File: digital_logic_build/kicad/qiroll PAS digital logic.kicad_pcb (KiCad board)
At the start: 2 copper layers, 49.5 x 32.4 mm, 47 parts, among them J2 led_sw1, J3 accessory, J4 mode_thr_batt, J5 3_pin, U1 4093B, U2 4027B, U3 4093B, U5 4093B, U6 14538B, U7 MCP1799_3V3

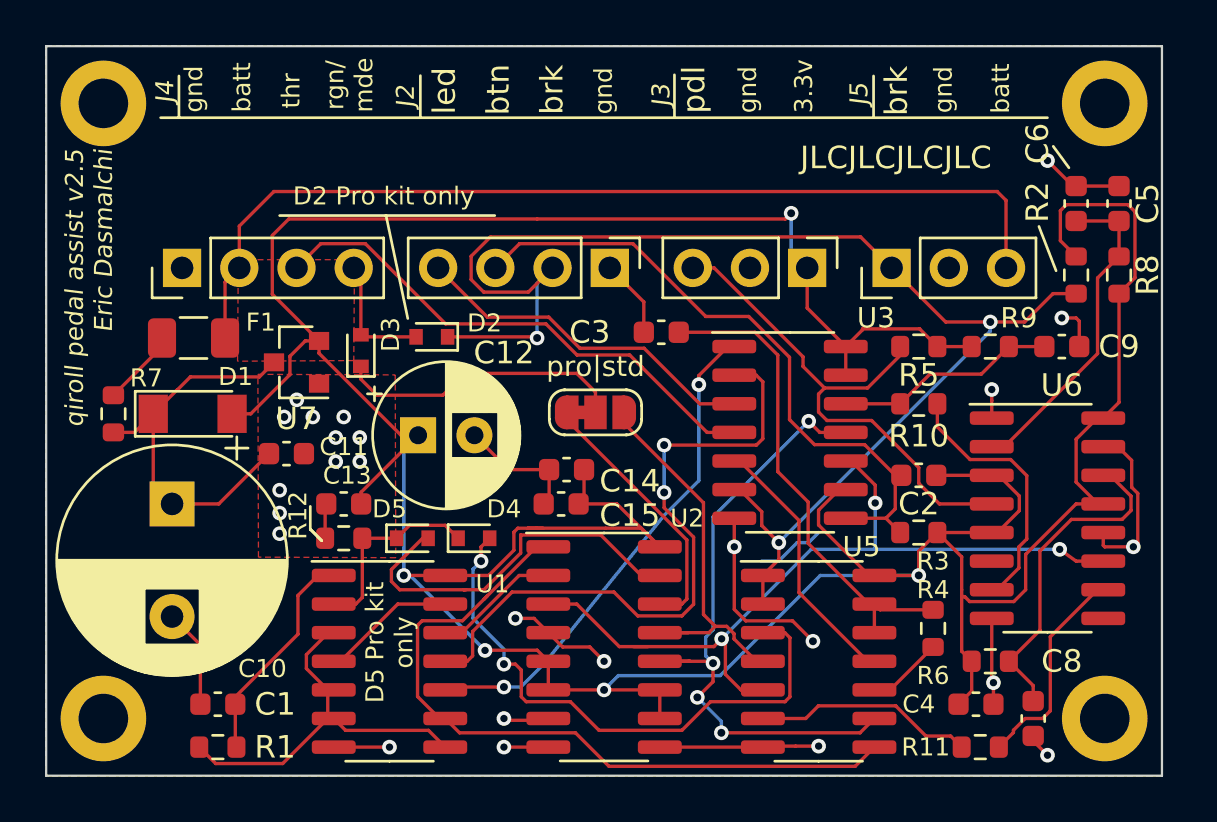
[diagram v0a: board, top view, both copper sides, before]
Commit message: add simple, update main pcb to KiCad 6
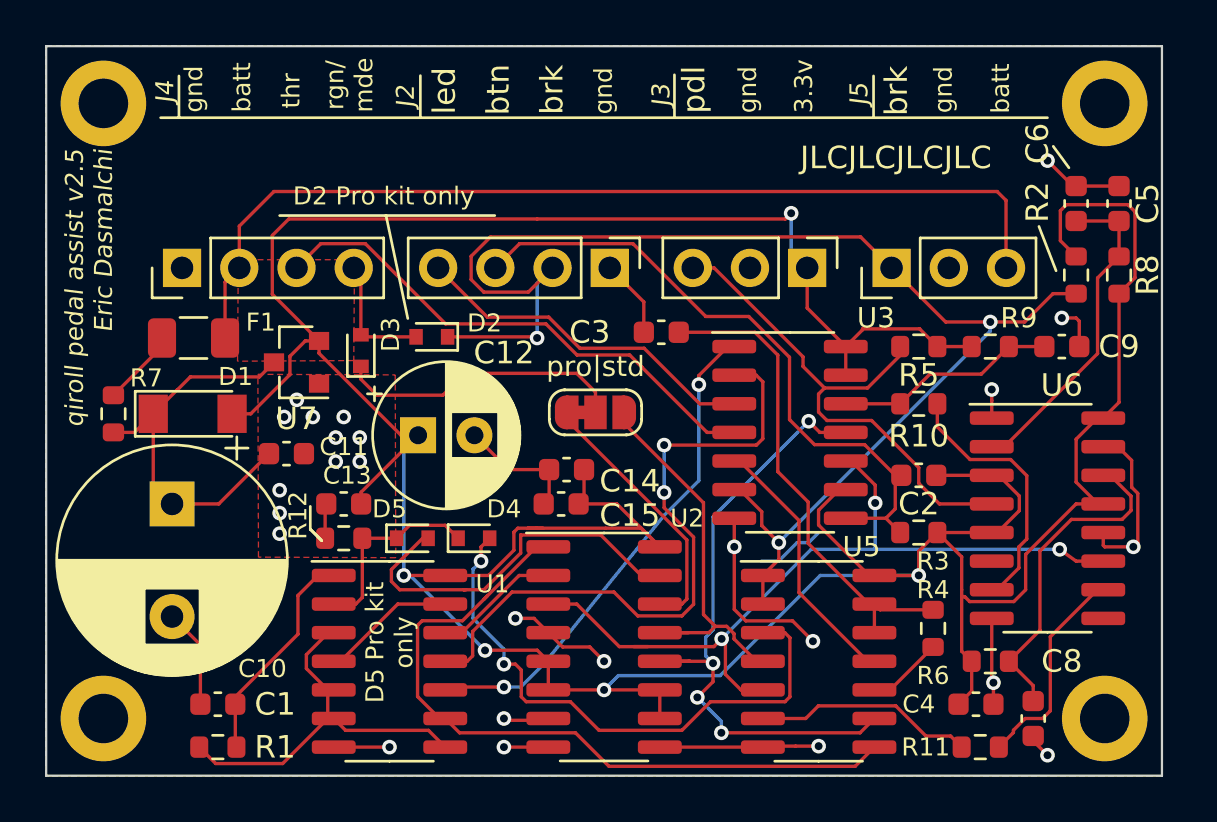
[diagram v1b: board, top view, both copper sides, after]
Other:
- net class Default removed
